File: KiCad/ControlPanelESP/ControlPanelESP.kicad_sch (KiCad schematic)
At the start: 41 parts, among them J1 Conn_01x02_Male, J2 Conn_01x06_Male, J3 Conn_01x04_Male, J4 Conn_01x03_Male, J5 Conn_01x02_Male, J6 Conn_01x04_Male, J7 Conn_01x02_Male, K1 DIPxx-1Axx-11x, Q1 Q_NPN_BEC, Q2 Q_NPN_BEC, Q3 Q_NMOS_GSD, Q4 Q_NMOS_GSD, Q5 Q_NMOS_GSD, SW1 SW_Push, SW2 SW_Push, U1 AMS1117-3.3, U2 ESP32-WROOM-32U, U3 LTV-817

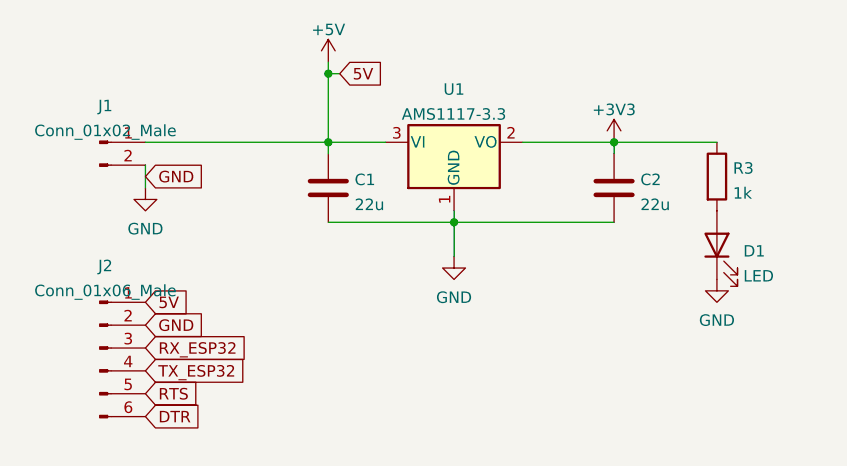
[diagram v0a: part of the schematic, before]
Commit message: second version
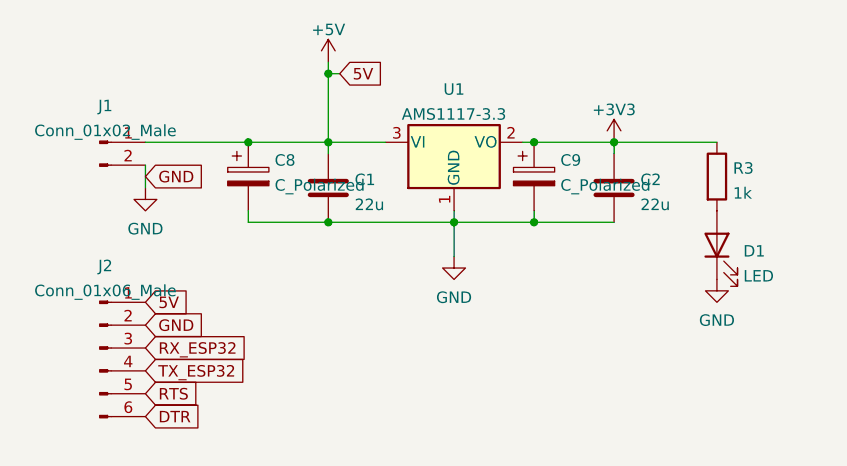
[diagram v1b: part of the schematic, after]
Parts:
- added C8, C9: C_Polarized, Capacitor_THT:CP_Radial_D5.0mm_P2.00mm, symbol Device:C_Polarized
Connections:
- net +3V3: now also C9.1
- net +5V: now also C8.1
- net GND: now also C8.2, C9.2
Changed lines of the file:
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@@
   (junction (at 34.29 139.7) (diameter 0) (color 0 0 0 0)
   )
+  (junction (at 46.99 39.37) (diameter 0) (color 0 0 0 0)
+  )
   (junction (at 223.52 128.27) (diameter 0) (color 0 0 0 0)
   )
   (junction (at 210.82 54.61) (diameter 0) (color 0 0 0 0)
   )
+  (junction (at 69.85 39.37) (diameter 0) (color 0 0 0 0)
+  )
   (junction (at 60.96 182.88) (diameter 0) (color 0 0 0 0)
   )
@@
   (junction (at 139.7 176.53) (diameter 0) (color 0 0 0 0)
   )
+  (junction (at 38.1 30.48) (diameter 0) (color 0 0 0 0)
+  )
+  (junction (at 69.85 30.48) (diameter 0) (color 0 0 0 0)
+  )
   (junction (at 24.13 165.1) (diameter 0) (color 0 0 0 0)
   )
@@
     (stroke (width 0) (type default) (color 0 0 0 0))
   )
+  (wire (pts (xy 38.1 30.48) (xy 46.99 30.48))
+    (stroke (width 0) (type default) (color 0 0 0 0))
+  )
+  (wire (pts (xy 69.85 39.37) (xy 78.74 39.37))
+    (stroke (width 0) (type default) (color 0 0 0 0))
+  )
   (wire (pts (xy 46.99 125.73) (xy 46.99 129.54))
     (stroke (width 0) (type default) (color 0 0 0 0))
@@
     (stroke (width 0) (type default) (color 0 0 0 0))
   )
+  (wire (pts (xy 69.85 30.48) (xy 78.74 30.48))
+    (stroke (width 0) (type default) (color 0 0 0 0))
+  )
   (wire (pts (xy 97.79 175.26) (xy 97.79 167.64))
     (stroke (width 0) (type default) (color 0 0 0 0))
@@
     (stroke (width 0) (type default) (color 0 0 0 0))
   )
-  (wire (pts (xy 60.96 39.37) (xy 78.74 39.37))
+  (wire (pts (xy 60.96 39.37) (xy 69.85 39.37))
     (stroke (width 0) (type default) (color 0 0 0 0))
   )
@@
     (stroke (width 0) (type default) (color 0 0 0 0))
   )
-  (wire (pts (xy 68.58 30.48) (xy 78.74 30.48))
+  (wire (pts (xy 68.58 30.48) (xy 69.85 30.48))
     (stroke (width 0) (type default) (color 0 0 0 0))
   )
@@
     (stroke (width 0) (type default) (color 0 0 0 0))
   )
+  (wire (pts (xy 38.1 38.1) (xy 38.1 39.37))
+    (stroke (width 0) (type default) (color 0 0 0 0))
+  )
   (wire (pts (xy 210.82 54.61) (xy 210.82 44.45))
     (stroke (width 0) (type default) (color 0 0 0 0))
@@
     (stroke (width 0) (type default) (color 0 0 0 0))
   )
+  (wire (pts (xy 38.1 39.37) (xy 46.99 39.37))
+    (stroke (width 0) (type default) (color 0 0 0 0))
+  )
   (wire (pts (xy 218.44 128.27) (xy 223.52 128.27))
     (stroke (width 0) (type default) (color 0 0 0 0))
   )
-  (wire (pts (xy 26.67 30.48) (xy 46.99 30.48))
+  (wire (pts (xy 26.67 30.48) (xy 38.1 30.48))
     (stroke (width 0) (type default) (color 0 0 0 0))
   )
@@
   )
   (polyline (pts (xy 15.24 111.76) (xy 105.41 111.76))
+    (stroke (width 0) (type default) (color 0 0 0 0))
+  )
+  (wire (pts (xy 69.85 38.1) (xy 69.85 39.37))
     (stroke (width 0) (type default) (color 0 0 0 0))
   )
@@
     (pin "2")
   )
+  (symbol (lib_id "Device:C_Polarized") (at 69.85 34.29 0) (unit 1)
+    (in_bom yes) (on_board yes) (fields_autoplaced)
+    (property "Reference" "C9" (id 0) (at 72.771 32.4925 0)
+      (effects (font (size 1.27 1.27)) (justify left))
+    )
+    (property "Value" "C_Polarized" (id 1) (at 72.771 35.2676 0)
+      (effects (font (size 1.27 1.27)) (justify left))
+    )
+    (property "Footprint" "Capacitor_THT:CP_Radial_D5.0mm_P2.00mm" (id 2) (at 70.8152 38.1 0)
+      (effects (font (size 1.27 1.27)) hide)
+    )
+    (property "Datasheet" "~" (id 3) (at 69.85 34.29 0)
+      (effects (font (size 1.27 1.27)) hide)
+    )
+    (pin "1")
+    (pin "2")
+  )
   (symbol (lib_id "power:+5V") (at 231.14 106.68 0) (unit 1)
     (in_bom yes) (on_board yes) (fields_autoplaced)
@@
     (pin "1")
   )
+  (symbol (lib_id "Device:C_Polarized") (at 38.1 34.29 0) (unit 1)
+    (in_bom yes) (on_board yes) (fields_autoplaced)
+    (property "Reference" "C8" (id 0) (at 41.021 32.4925 0)
+      (effects (font (size 1.27 1.27)) (justify left))
+    )
+    (property "Value" "C_Polarized" (id 1) (at 41.021 35.2676 0)
+      (effects (font (size 1.27 1.27)) (justify left))
+    )
+    (property "Footprint" "Capacitor_THT:CP_Radial_D5.0mm_P2.00mm" (id 2) (at 39.0652 38.1 0)
+      (effects (font (size 1.27 1.27)) hide)
+    )
+    (property "Datasheet" "~" (id 3) (at 38.1 34.29 0)
+      (effects (font (size 1.27 1.27)) hide)
+    )
+    (pin "1")
+    (pin "2")
+  )
   (symbol (lib_id "Device:C") (at 46.99 35.56 0) (unit 1)
     (in_bom yes) (on_board yes) (fields_autoplaced)
@@
       (reference "C7") (unit 1) (value "100n") (footprint "Capacitor_SMD:C_0805_2012Metric_Pad1.18x1.45mm_HandSolder")
     )
+    (path "/fb12d38d-9b26-4e6c-9a22-280965560e28"
+      (reference "C8") (unit 1) (value "C_Polarized") (footprint "Capacitor_THT:CP_Radial_D5.0mm_P2.00mm")
+    )
+    (path "/cd0e1ec8-5612-4244-a876-838286424de9"
+      (reference "C9") (unit 1) (value "C_Polarized") (footprint "Capacitor_THT:CP_Radial_D5.0mm_P2.00mm")
+    )
     (path "/3cacc5b5-0b9a-41df-a427-24c30f1eb6f8"

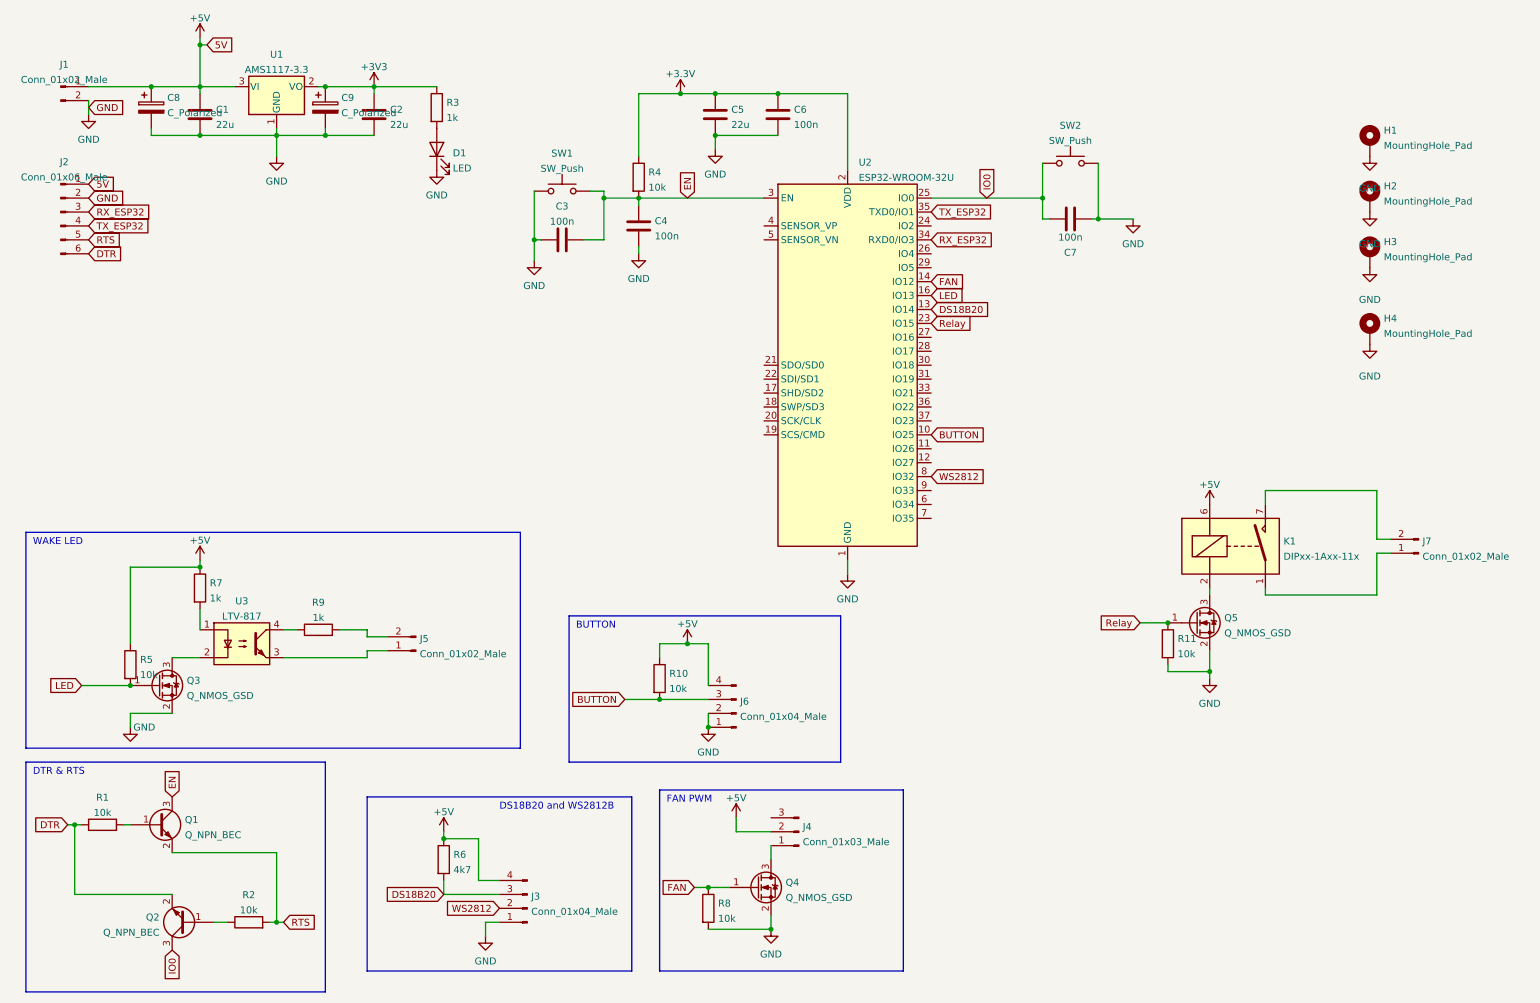
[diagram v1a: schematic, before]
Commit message: V2.0 of PCB
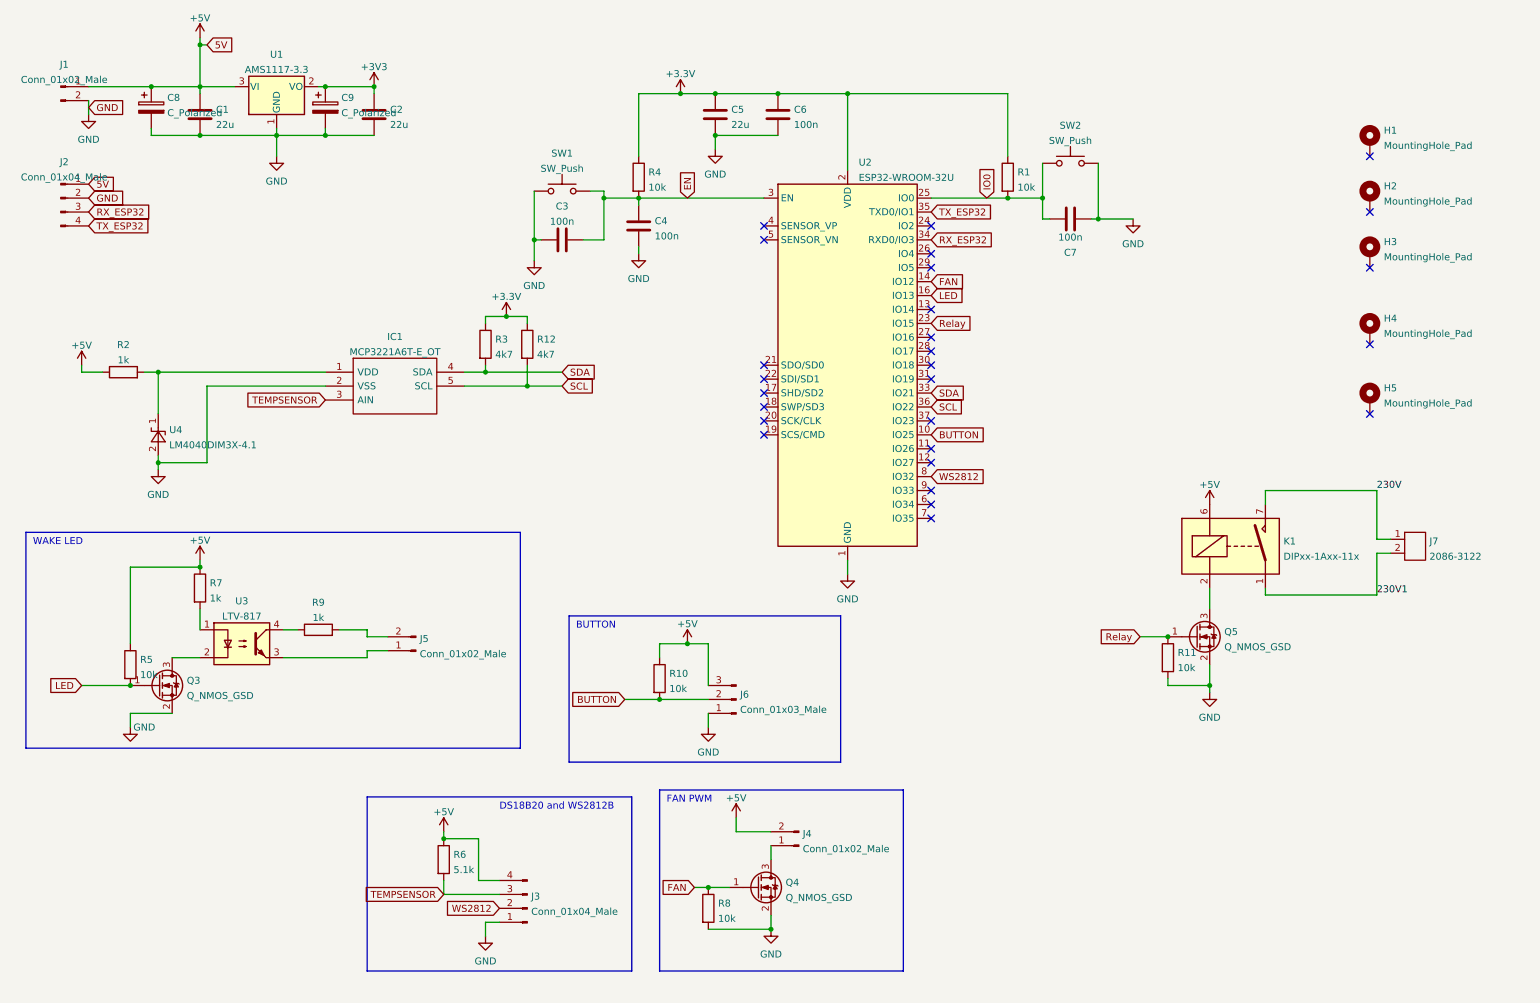
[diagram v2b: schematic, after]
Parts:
- removed D1: LED, LED_SMD:LED_0805_2012Metric_Pad1.15x1.40mm_HandSolder, symbol Device:LED
- removed J2: Conn_01x06_Male, Connector_JST:JST_XH_B6B-XH-A_1x06_P2.50mm_Vertical, symbol Connector:Conn_01x06_Male
- removed J4: Conn_01x03_Male, Connector_JST:JST_XH_B3B-XH-A_1x03_P2.50mm_Vertical, symbol Connector:Conn_01x03_Male
- removed J6: Conn_01x04_Male, symbol Connector:Conn_01x04_Male
- removed J7: Conn_01x02_Male, Connector_JST:JST_XH_B2B-XH-A_1x02_P2.50mm_Vertical, symbol Connector:Conn_01x02_Male
- removed Q1, Q2: Q_NPN_BEC, Package_TO_SOT_SMD:SOT-23, symbol Device:Q_NPN_BEC
- added H5: MountingHole_Pad, MountingHole:MountingHole_2.2mm_M2_DIN965_Pad, symbol Mechanical:MountingHole_Pad
- added IC1: MCP3221A6T-E_OT, SOT95P280X145-5N, symbol SamacSys_Parts:MCP3221A6T-E_OT
- added J2: Conn_01x04_Male, Connector_PinHeader_2.54mm:PinHeader_1x04_P2.54mm_Vertical, symbol Connector:Conn_01x04_Male
- added J4: Conn_01x02_Male, Connector_PinHeader_2.54mm:PinHeader_1x02_P2.54mm_Vertical, symbol Connector:Conn_01x02_Male
- added J6: Conn_01x03_Male, Connector_PinHeader_2.54mm:PinHeader_1x03_P2.54mm_Vertical, symbol Connector:Conn_01x03_Male
- added J7: 2086-3122, Lichtwecker:2086-3122, symbol Lichtwecker_Symbols:2086-3122
- added R12: 4k7, Resistor_SMD:R_0805_2012Metric_Pad1.20x1.40mm_HandSolder, symbol Device:R
- added U4: LM4040DIM3X-4.1, Package_TO_SOT_SMD:SOT-23, symbol Lichtwecker_Symbols:LM4040DIM3X-4.1
- J1, J5: footprint Connector_JST:JST_XH_B2B-XH-A_1x02_P2.50mm_Vertical -> Connector_PinHeader_2.54mm:PinHeader_1x02_P2.54mm_Vertical
- J3: footprint (none) -> Connector_PinHeader_2.54mm:PinHeader_1x04_P2.54mm_Vertical
- R2: value 10k -> 1k
- R3: value 1k -> 4k7
- R6: value 4k7 -> 5.1k
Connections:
- net DTR is gone; now on net +3V3: R1.1
- net +3V3: now also R12.1
- net +5V: now also R2.1, J2.1 (Pin_1), J4.2 (Pin_2), J6.3 (Pin_3)
- net BUTTON: now also J6.2 (Pin_2)
- net GND: now also IC1.2 (VSS), J2.2 (Pin_2), J6.1 (Pin_1), U4.2 (A); no longer H1.1, H2.1, H3.1, H4.1
- net IO0: now also R1.2
- net RX_ESP32: now also J2.3 (Pin_3)
- net TX_ESP32: now also J2.4 (Pin_4)
- net at Q4.3 (D): now also J4.1 (Pin_1)
- net SDA: now reaches U2.33 (IO21)
- net SDA: now also R3.2, IC1.4 (SDA)
- net SCL: now reaches U2.36 (IO22)
- net SCL: now also IC1.5 (SCL), R12.2
- net 230V1: now reaches K1.1, K1.14
- net 230V1: now also J7.2
- net 230V: now reaches K1.7, K1.8
- net 230V: now also J7.1
- net DS18B20 renamed TEMPSENSOR
- net TEMPSENSOR: now also IC1.3 (AIN); no longer U2.13 (IO14)
- net RTS: no longer names the net of R2.2
- net RTS: now also IC1.1 (VDD), U4.1 (K)
- no-connect marks 0 -> 27
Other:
- note removed: "DTR & RTS"
- moved on the sheet: Q5, R11
